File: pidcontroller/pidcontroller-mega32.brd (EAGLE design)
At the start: 100 x 75.4 mm, 32 parts, among them IC2 MAX3232CWE, IC3 MEGA32-A

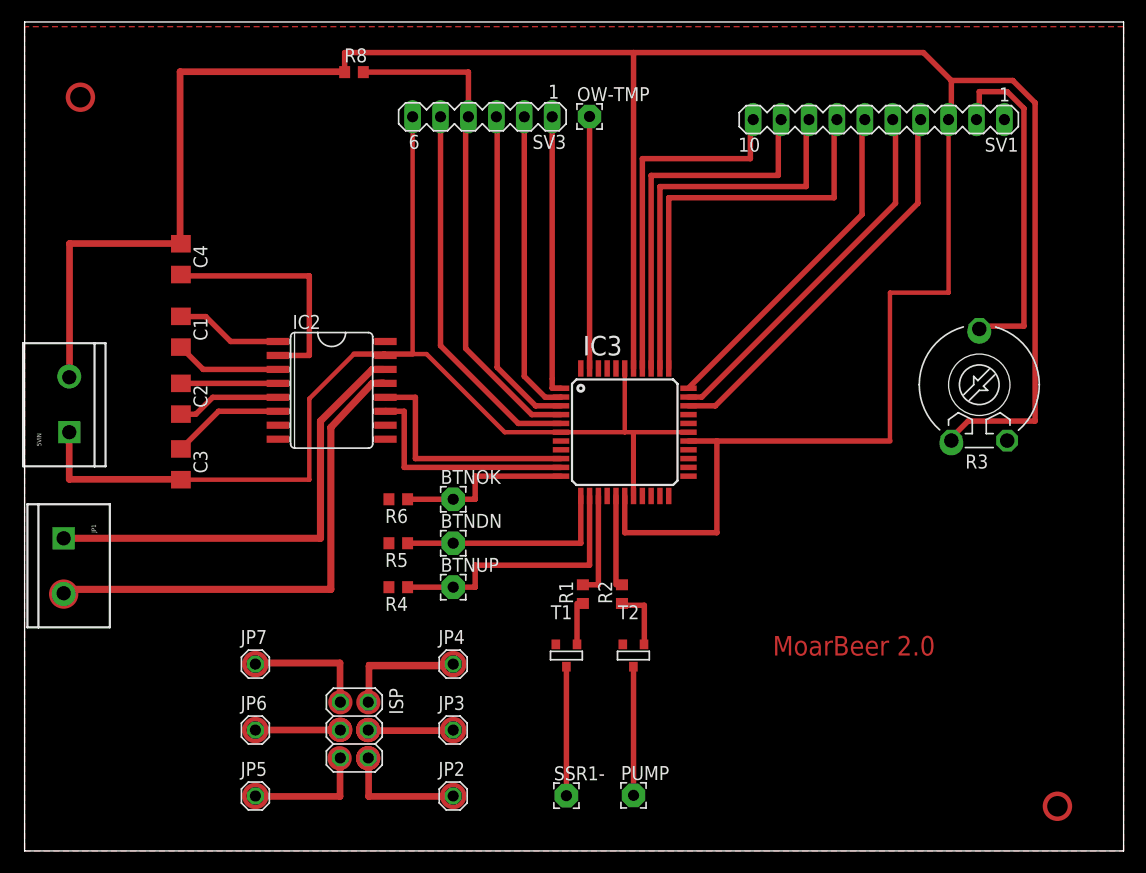
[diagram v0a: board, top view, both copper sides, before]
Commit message: changed stuff
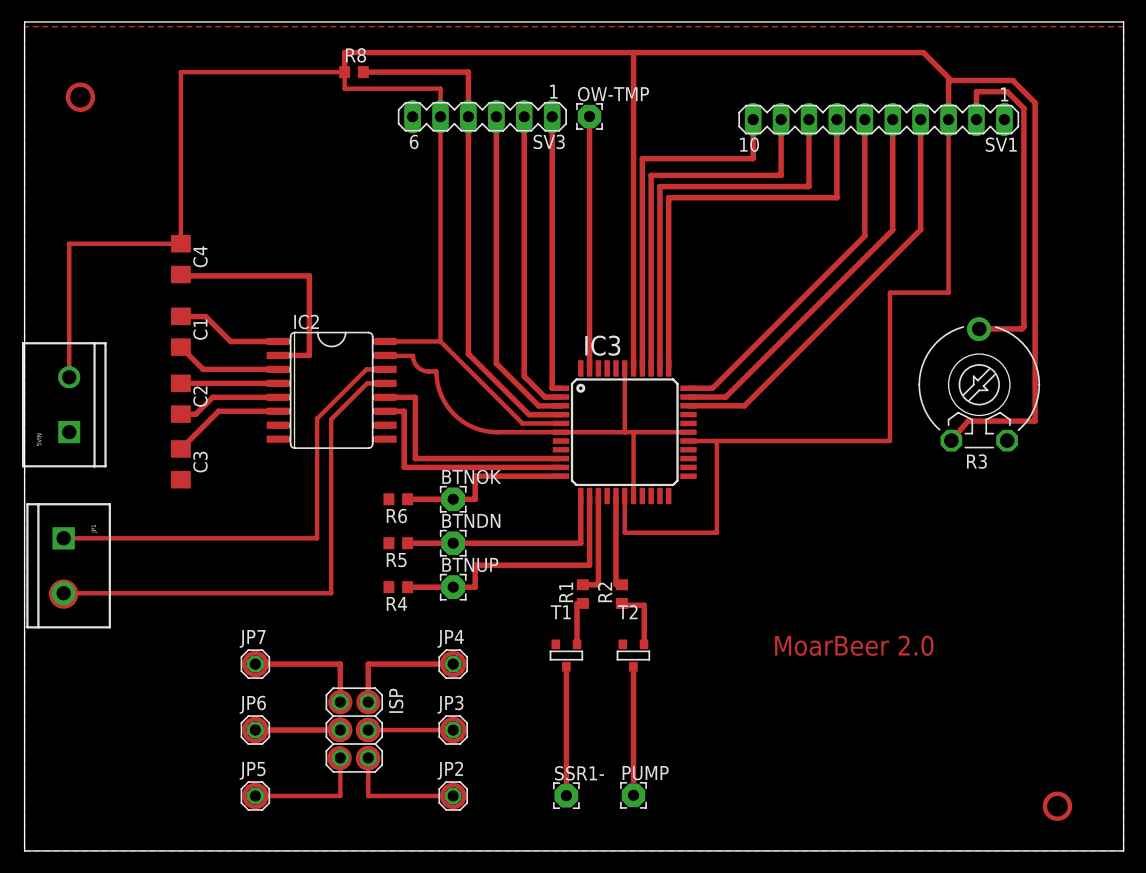
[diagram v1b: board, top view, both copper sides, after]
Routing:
- net GND: track 111.9 -> 42.1 mm
- net N$39: track 45.2 -> 0.00 mm
- net N$30: track 30.0 -> 0.00 mm
- net N$29: track 22.0 -> 0.00 mm
- net VCC: track 299.7 -> 314.6 mm, vias 1 -> 0
- net N$31: track 14.1 -> 0.00 mm
- net N$37: track 11.4 -> 0.00 mm
- net N$35: track 11.1 -> 0.00 mm
- net N$34: track 11.1 -> 0.00 mm
- net N$32: track 10.1 -> 0.00 mm
- net N$36: track 7.67 -> 0.06 mm
- net N$33: track 7.55 -> 0.00 mm, vias 0 -> 1
- net D7: track 36.2 -> 37.8 mm
- net D5: track 31.2 -> 32.4 mm
- net D6: track 33.9 -> 34.9 mm
